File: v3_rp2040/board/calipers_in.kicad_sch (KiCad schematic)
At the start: 14 parts, among them IC1 LM393, J9 USB_A, U12 USBLC6-2SC6

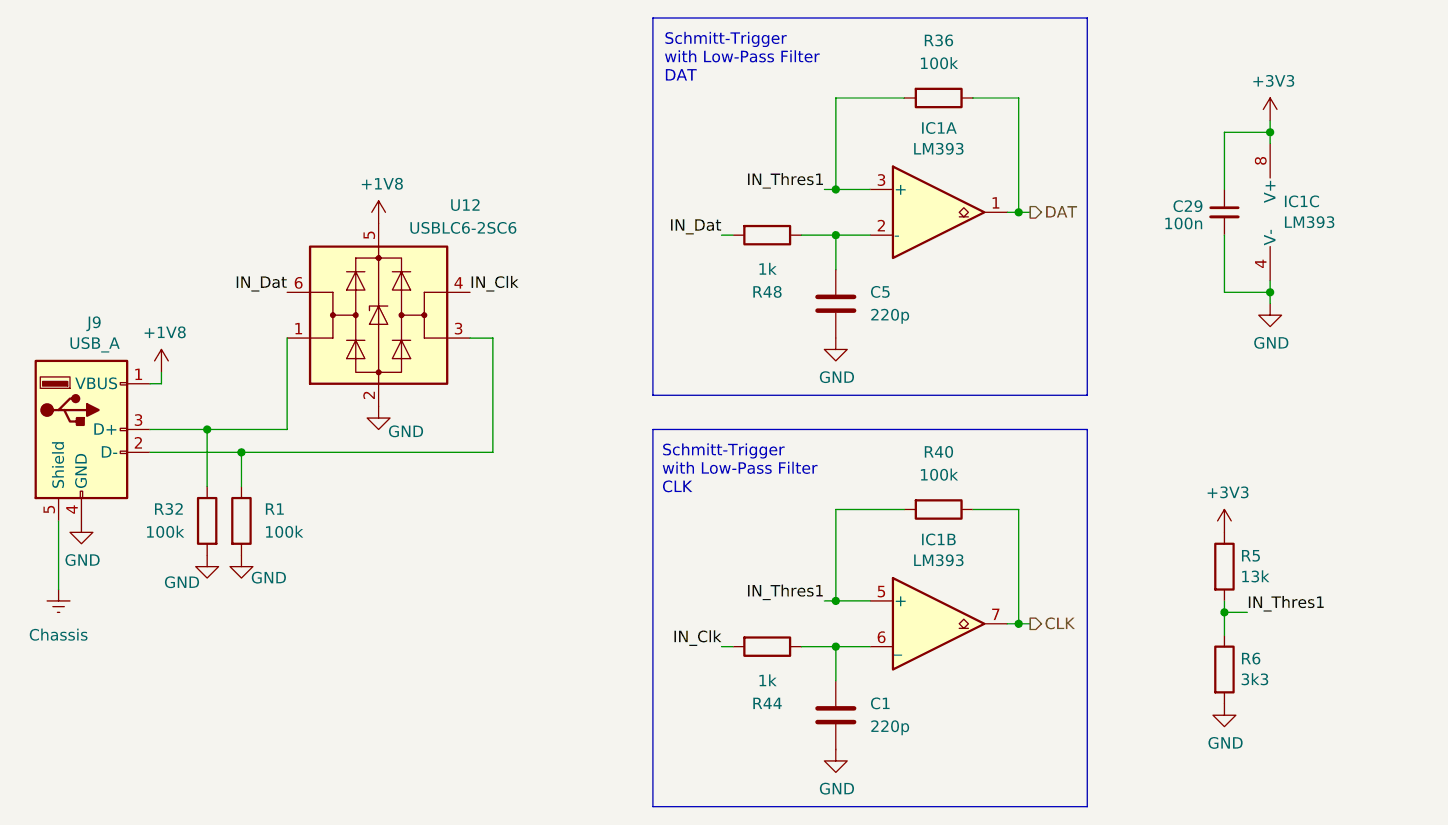
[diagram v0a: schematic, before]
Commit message: more schematic work
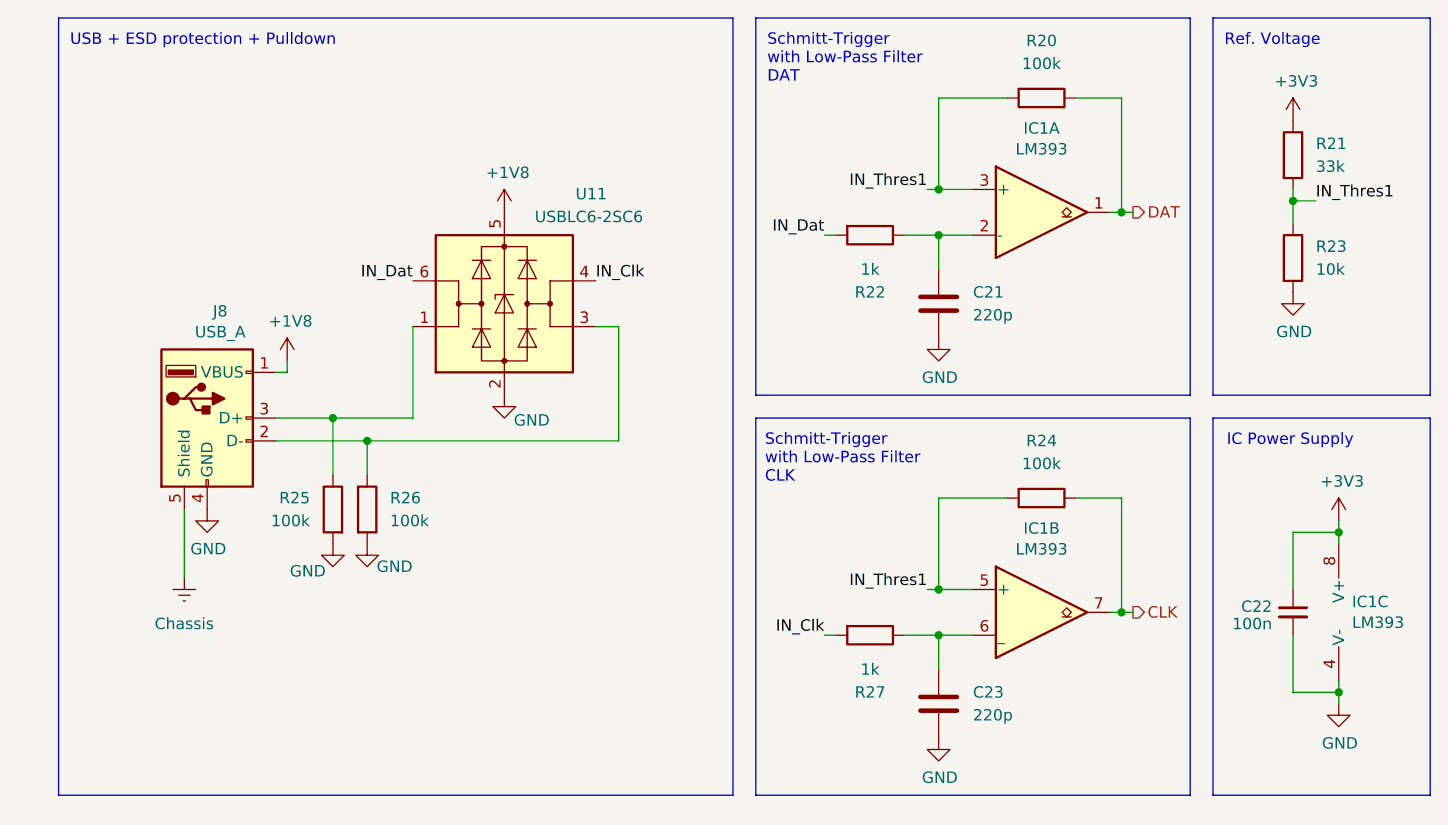
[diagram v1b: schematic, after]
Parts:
- removed R5: 13k, Resistor_SMD:R_0603_1608Metric, symbol Device:R
- removed R6: 3k3, Resistor_SMD:R_0603_1608Metric, symbol Device:R
- added R21: 33k, Resistor_SMD:R_0402_1005Metric, symbol Device:R
- added R23: 10k, Resistor_SMD:R_0402_1005Metric, symbol Device:R
- renumbered C5 to C21, C29 to C22, C1 to C23, J9 to J8, R36 to R20, R48 to R22, R40 to R24, R32 to R25, R1 to R26, R44 to R27, U12 to U11
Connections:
- net +3V3: now also R21.1
- net GND: now also R23.2
- net IN_Thres1: now also R21.2, R23.1
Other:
- note added: "IC Power Supply"
- note added: "Ref. Voltage"
- note added: "USB + ESD protection + Pulldown"
- moved on the sheet: C21, C22, C23, IC1A, IC1B, IC1C, J8, R20, R22, R24, R25, R26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
